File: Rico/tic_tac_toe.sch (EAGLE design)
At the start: 18 parts, among them IC1 PCF8574P, U1 ATMEGA328P_PDIP

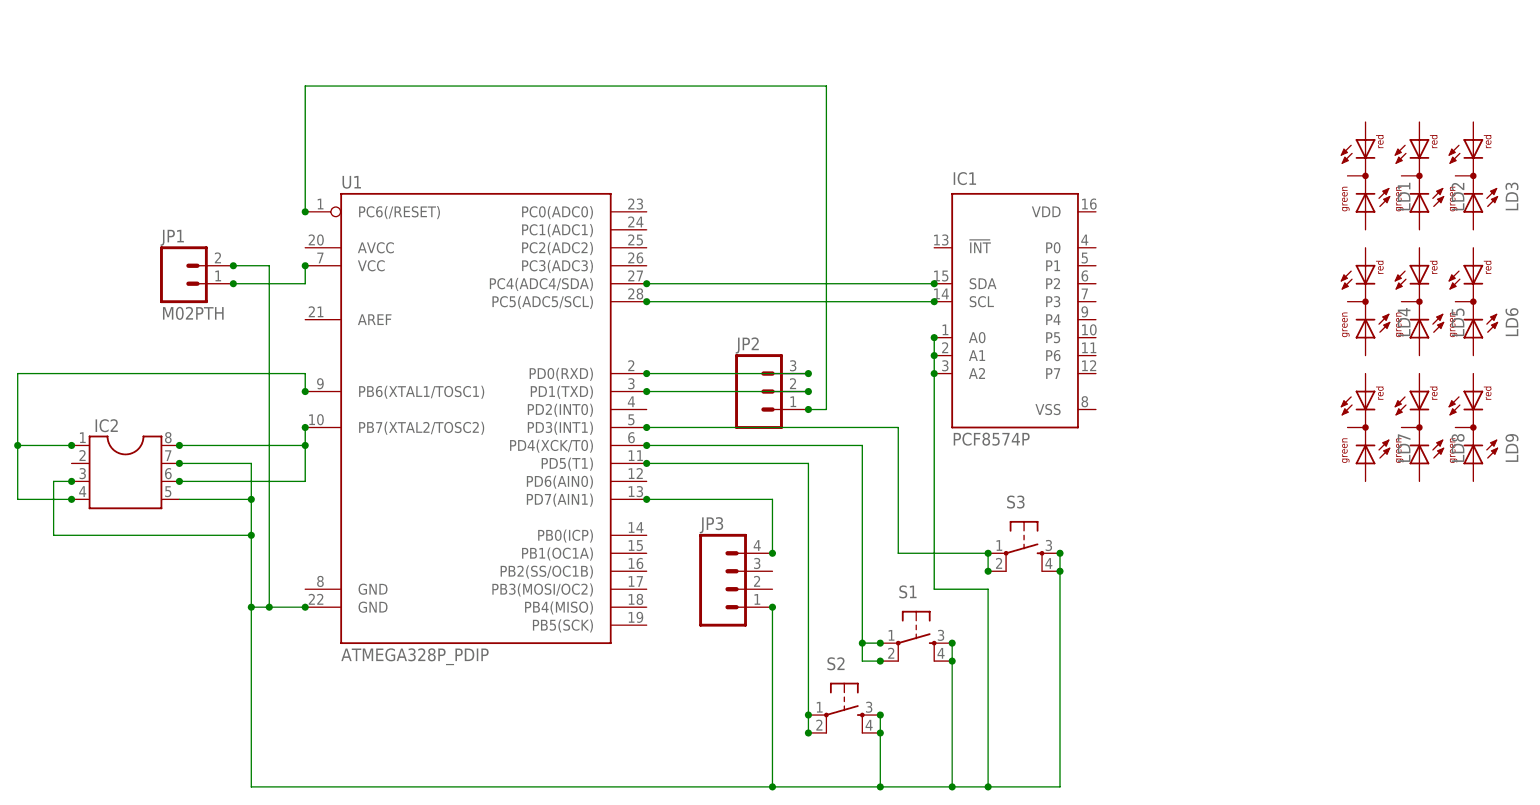
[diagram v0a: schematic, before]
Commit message: ricoh: almost finish schematic, add board, route.
* schematic: PCF VCC and GND are still switched up (fixed in brd)
* board: ready for review.
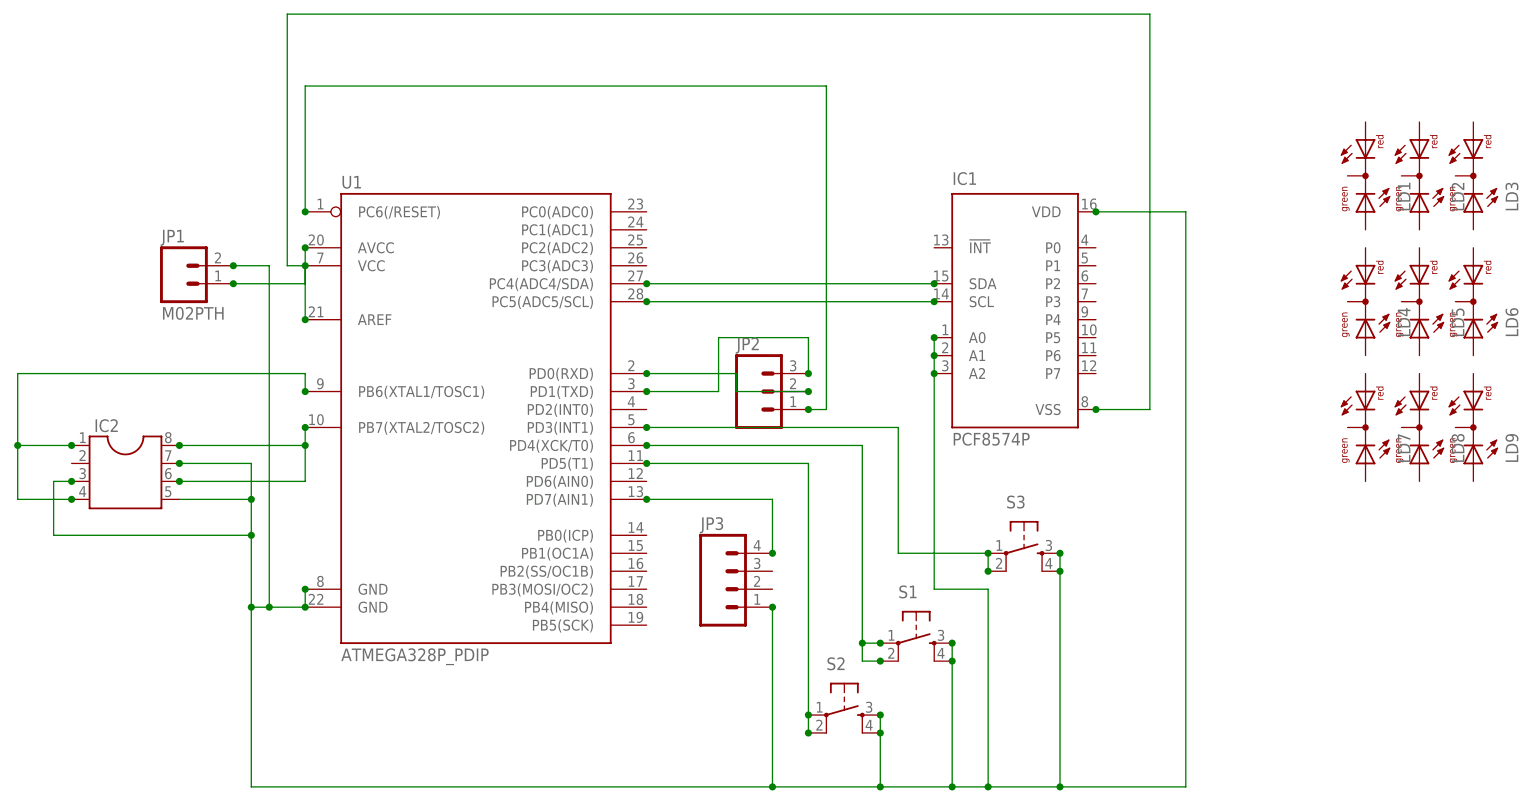
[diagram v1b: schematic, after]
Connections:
- net GND: now also IC1.VDD, U1.GND@1
- net RX: now also JP2.2; no longer JP2.3
- net TX: now also JP2.3; no longer JP2.2
- net VCC: now also IC1.VSS, U1.AREF, U1.AVCC
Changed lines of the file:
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@@
 <junction x="-12.7" y="68.58"/>
 <junction x="-2.54" y="71.12"/>
+<pinref part="IC1" gate="G$1" pin="VSS"/>
+<wire x1="109.22" y1="50.8" x2="116.84" y2="50.8" width="0.1524" layer="91"/>
+<wire x1="116.84" y1="50.8" x2="116.84" y2="106.68" width="0.1524" layer="91"/>
+<wire x1="116.84" y1="106.68" x2="-5.08" y2="106.68" width="0.1524" layer="91"/>
+<wire x1="-5.08" y1="106.68" x2="-5.08" y2="71.12" width="0.1524" layer="91"/>
+<wire x1="-5.08" y1="71.12" x2="-2.54" y2="71.12" width="0.1524" layer="91"/>
+<junction x="109.22" y="50.8"/>
+<pinref part="U1" gate="G$1" pin="AVCC"/>
+<wire x1="-2.54" y1="73.66" x2="-2.54" y2="71.12" width="0.1524" layer="91"/>
+<pinref part="U1" gate="G$1" pin="AREF"/>
+<wire x1="-2.54" y1="63.5" x2="-2.54" y2="71.12" width="0.1524" layer="91"/>
+<junction x="-2.54" y="73.66"/>
+<junction x="-2.54" y="63.5"/>
 </segment>
 </net>
@@
 <junction x="63.5" y="-2.54"/>
 <junction x="63.5" y="22.86"/>
+<pinref part="IC1" gate="G$1" pin="VDD"/>
+<wire x1="109.22" y1="78.74" x2="121.92" y2="78.74" width="0.1524" layer="91"/>
+<wire x1="121.92" y1="78.74" x2="121.92" y2="-2.54" width="0.1524" layer="91"/>
+<wire x1="121.92" y1="-2.54" x2="104.14" y2="-2.54" width="0.1524" layer="91"/>
+<junction x="104.14" y="-2.54"/>
+<junction x="109.22" y="78.74"/>
+<pinref part="U1" gate="G$1" pin="GND@1"/>
+<wire x1="-2.54" y1="22.86" x2="-2.54" y2="25.4" width="0.1524" layer="91"/>
+<junction x="-2.54" y="25.4"/>
 </segment>
 </net>
@@
 </segment>
 </net>
-<net name="RX" class="0">
-<segment>
-<pinref part="JP2" gate="G$1" pin="3"/>
-<pinref part="U1" gate="G$1" pin="PD0(RXD)"/>
-<wire x1="68.58" y1="55.88" x2="45.72" y2="55.88" width="0.1524" layer="91"/>
-<junction x="68.58" y="55.88"/>
-<junction x="45.72" y="55.88"/>
-</segment>
-</net>
-<net name="TX" class="0">
-<segment>
-<pinref part="JP2" gate="G$1" pin="2"/>
-<pinref part="U1" gate="G$1" pin="PD1(TXD)"/>
-<wire x1="68.58" y1="53.34" x2="45.72" y2="53.34" width="0.1524" layer="91"/>
-<junction x="68.58" y="53.34"/>
-<junction x="45.72" y="53.34"/>
-</segment>
-</net>
 <net name="RESET" class="0">
 <segment>
@@
 </segment>
 </net>
+<net name="TX" class="0">
+<segment>
+<pinref part="U1" gate="G$1" pin="PD1(TXD)"/>
+<wire x1="45.72" y1="53.34" x2="55.88" y2="53.34" width="0.1524" layer="91"/>
+<wire x1="55.88" y1="53.34" x2="55.88" y2="60.96" width="0.1524" layer="91"/>
+<pinref part="JP2" gate="G$1" pin="3"/>
+<wire x1="55.88" y1="60.96" x2="68.58" y2="60.96" width="0.1524" layer="91"/>
+<wire x1="68.58" y1="60.96" x2="68.58" y2="55.88" width="0.1524" layer="91"/>
+<junction x="45.72" y="53.34"/>
+<junction x="68.58" y="55.88"/>
+</segment>
+</net>
+<net name="RX" class="0">
+<segment>
+<pinref part="U1" gate="G$1" pin="PD0(RXD)"/>
+<wire x1="45.72" y1="55.88" x2="58.42" y2="55.88" width="0.1524" layer="91"/>
+<wire x1="58.42" y1="55.88" x2="58.42" y2="53.34" width="0.1524" layer="91"/>
+<pinref part="JP2" gate="G$1" pin="2"/>
+<wire x1="58.42" y1="53.34" x2="68.58" y2="53.34" width="0.1524" layer="91"/>
+<junction x="45.72" y="55.88"/>
+<junction x="68.58" y="53.34"/>
+</segment>
+</net>
